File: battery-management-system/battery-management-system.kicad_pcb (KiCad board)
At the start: 4 copper layers, 100 x 111 mm, 212 parts, among them J1 CELL4_PLUS, J10 18V, J11 3V3, J12 AMPHENOL_micro_usb_10118194-0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, J13 I2C, J14 UART_INTERCONNECT, J15 LEDS, J16 CHARGE/DISCHARGE, J17 UART_USB, J18 rspro_header_5pin_3_5mm, J19 TEMP_CELL1, J2 CELL4_MINUS, J20 TEMP_CELL2, J21 TEMP_CELL3, J22 TEMP_CELL4, J23 Conn_01x05, J24 Charge, J25 Discharge, J3 CELL3_MINUS, J4 CELL2_MINUS, J5 CELL1_MINUS, J6 VBAT+, J7 VBAT+_CHARGE, J8 VBAT-, J9 5V, Q1 DMN3404L, Q10 DMN3404L, Q11 BS250FTA, Q12 BS250FTA, Q13 BS250FTA, Q14 BS250FTA, Q15 BS250FTA, Q16 DMN3404L, Q17 DMN3404L, Q18 DMN3404L, Q19 DMN3404L, Q2 TJ40S04M3L, Q20 DMN3404L, Q21 DMN3404L, Q22 DMN3404L, Q23 DMN3404L, Q24 DMN3404L, Q25 DMN3404L, Q26 DMN3404L, Q27 DMN3404L, Q28 DMN3404L, Q29 DMN3404L, Q3 TJ40S04M3L, Q30 DMN3404L, Q31 DMN3404L, Q32 DMN3404L, Q33 DMN3404L, Q34 DMN3404L, Q35 DMN3404L, Q36 DMN3404L, Q37 DMN3404L, Q38 DMN3404L, Q39 DMN3404L, Q4 DMN3404L, Q40 TJ40S04M3L, Q5 DMN3404L, Q6 DMN3404L, Q7 DMN3404L, Q8 DMN3404L, Q9 DMN3404L, U1 ICL7660, U10 STM32L071CZTx, U11 LM2904M8-13, U12 LM2904M8-13, U13 MC74VHC139, U2 L6982C33DR, U3 L6982C33DR, U4 ICL7660, U5 FT230XS, U6 ARM-JTAG-SWD, U7 AT24C512C, U8 NCT75DR2G, U9 STC3100

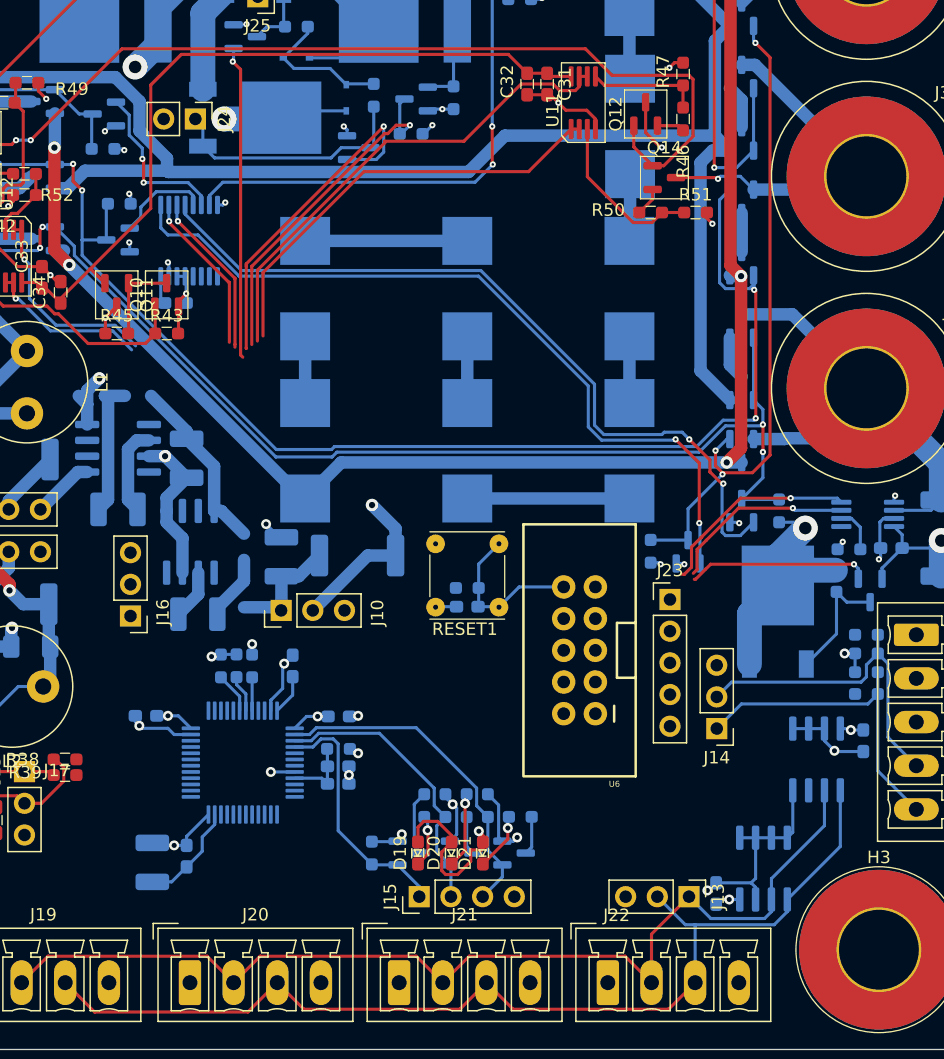
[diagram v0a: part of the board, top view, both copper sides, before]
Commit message: improve layout
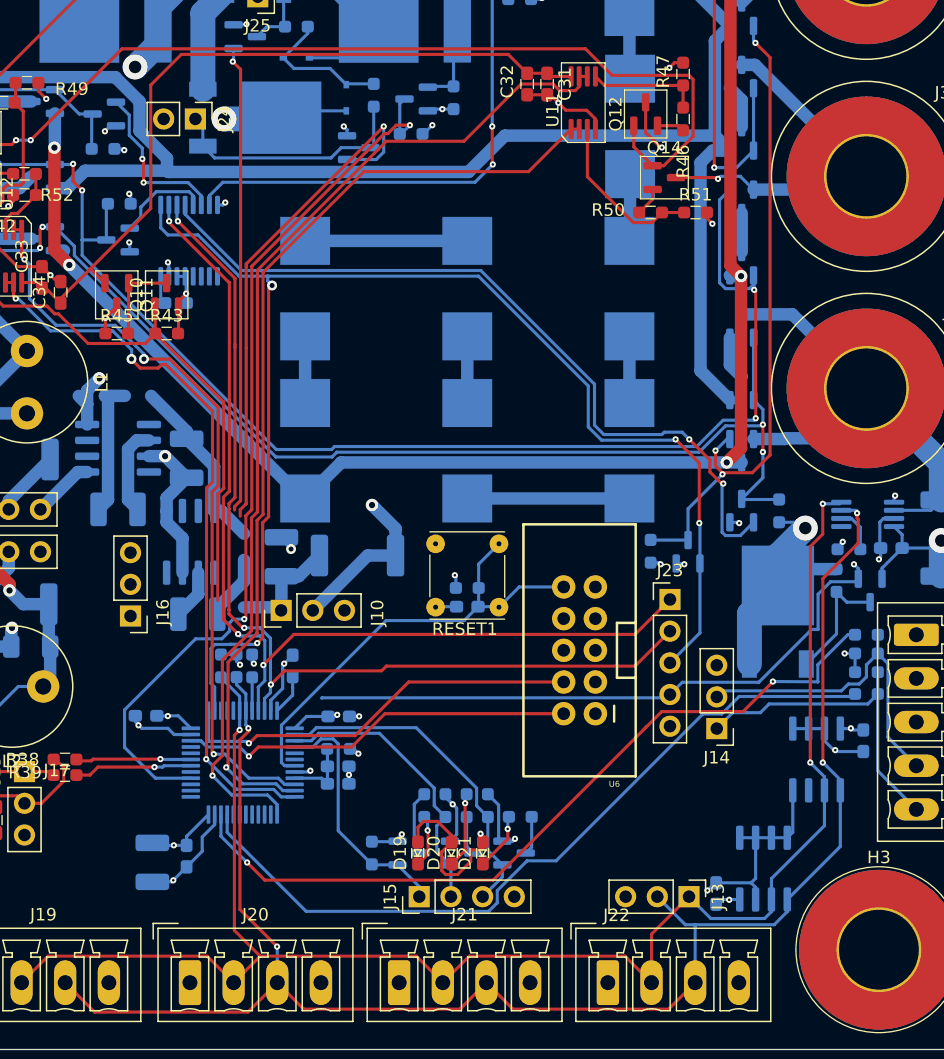
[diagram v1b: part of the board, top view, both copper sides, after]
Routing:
- net /CELL_BALANCING_A0: track 13.0 -> 80.1 mm, vias 1 -> 3
- net /CELL_BALANCING_A1: track 13.3 -> 78.8 mm, vias 1 -> 3
- net Net-(U10-PB11): track 0.00 -> 63.2 mm, vias 0 -> 2
- net Net-(U10-PB10): track 0.00 -> 62.2 mm
- net /CELL_BALANCING_STROBE: track 62.9 -> 110.9 mm, vias 2 -> 4
- net /Cell Measurement/CELL3: track 13.0 -> 58.7 mm, vias 1 -> 3
- net /Battery Pack/CHARGE_AVAILABLE: track 27.7 -> 72.3 mm, vias 1 -> 2
- net /Cell Measurement/CELL1: track 16.5 -> 60.9 mm, vias 1 -> 3
- net /Cell Measurement/CELL4: track 39.5 -> 82.8 mm, vias 0 -> 1
- net /Cell Measurement/CELL2: track 35.2 -> 77.3 mm, vias 0 -> 1
- net /EN_CELL_BALANCING: track 14.6 -> 50.0 mm
- net /MCU/SDA: track 101.9 -> 136.0 mm, vias 1 -> 4
- net /MCU/SWCLK: track 0.00 -> 33.0 mm, vias 0 -> 1
- net /MCU/SWDIO: track 0.00 -> 31.8 mm, vias 0 -> 1
- net /MCU/SCL: track 102.7 -> 132.5 mm, vias 1 -> 3
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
